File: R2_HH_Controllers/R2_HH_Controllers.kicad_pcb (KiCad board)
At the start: 4 copper layers, 55.6 x 111.3 mm, 122 parts, among them IC1 E22-900M22S, IC2 E22-900M22S, J1 USB4105-GF-A, J2 S2B-PH-SM4-TB_LF__SN_, J3 USB4105-GF-A, J4 S2B-PH-SM4-TB_LF__SN_, SW1 SW_Push, SW10 Boot, SW11 PCM12SMTR, SW12 SW_Push, SW13 SW_Push, SW14 SW_Push, SW15 SW_Push, SW16 SW_Push, SW17 SW_Push, SW18 SW_Push, SW19 SW_Push, SW2 SW_Push, SW20 Reset, SW21 Boot, SW22 PCM12SMTR, SW3 SW_Push, SW4 SW_Push, SW5 SW_Push, SW6 SW_Push, SW7 SW_Push, SW8 SW_Push, SW9 Reset, U1 AP2112K-3.3, U2 ESP32-S3-MINI-1, U3 BQ24074RGT, U4 USBLC6-2SC6, U5 AP2112K-3.3, U6 ESP32-S3-MINI-1, U7 BQ24074RGT, U8 USBLC6-2SC6

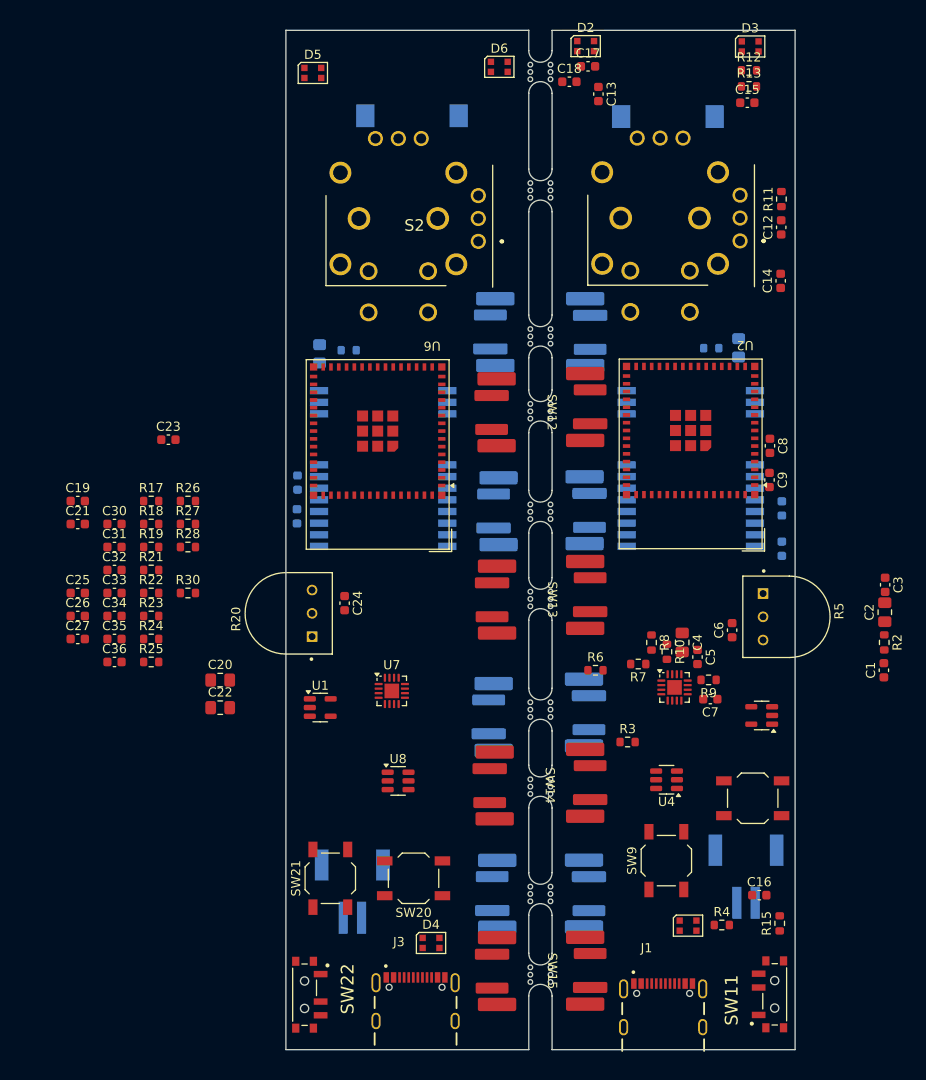
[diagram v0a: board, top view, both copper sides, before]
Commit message: updates
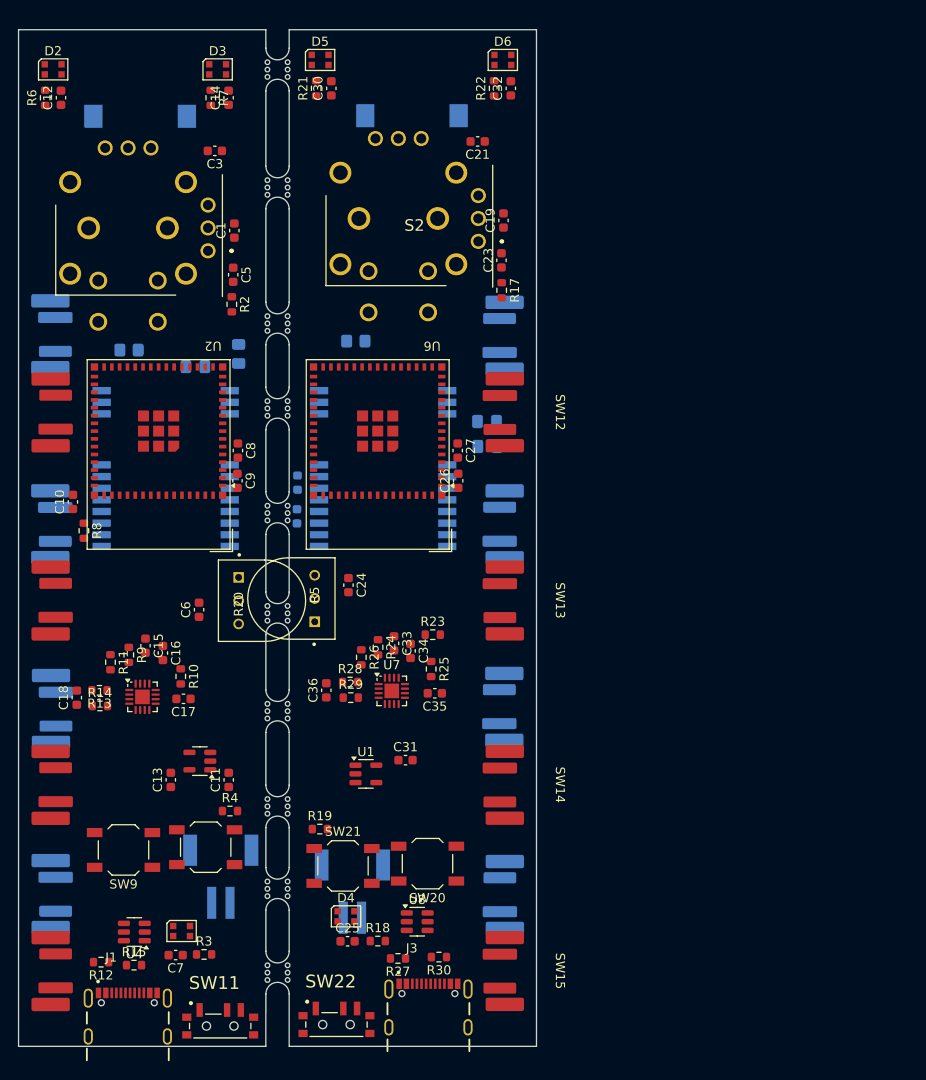
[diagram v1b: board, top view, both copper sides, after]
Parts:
- C10, C11, R14, R29: moved to F.Cu
- C2, C20, C22, C4: moved to B.Cu
- moved R12 120.3 mm to (132.5, 126.8), turned to 180 degrees
- moved R13 96.8 mm to (132.3, 97.1), turned to 180 degrees
- moved R11 89.0 mm to (133.5, 94.1), turned to -90 degrees
- moved C15 88.5 mm to (137.3, 92.3), turned to -90 degrees
- moved C13 88.2 mm to (140.1, 106.9), turned to 90 degrees
- moved C3 87.2 mm to (144.9, 38.2), turned to 180 degrees
- moved R6 86.7 mm to (126.4, 32.4), turned to 90 degrees
- moved C18 86.1 mm to (129.8, 97.9), turned to 90 degrees
- moved C1 85.6 mm to (147.0, 46.9)
- moved C17 82.0 mm to (141.5, 98.1), turned to 180 degrees
- moved R2 80.2 mm to (146.7, 55.0)
- moved C12 79.9 mm to (128.1, 32.4)
- moved C10 77.6 mm to (129.4, 76.6)
- moved R7 77.5 mm to (144.4, 32.4), turned to -90 degrees
- moved R14 77.3 mm to (132.3, 98.8)
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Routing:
- removed copper zone on In1.Cu, net GND
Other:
- board size 55.6 x 111.3 mm -> 56.5 x 111 mm
